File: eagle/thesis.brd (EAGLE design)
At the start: 99.1 x 60.2 mm, 14 parts

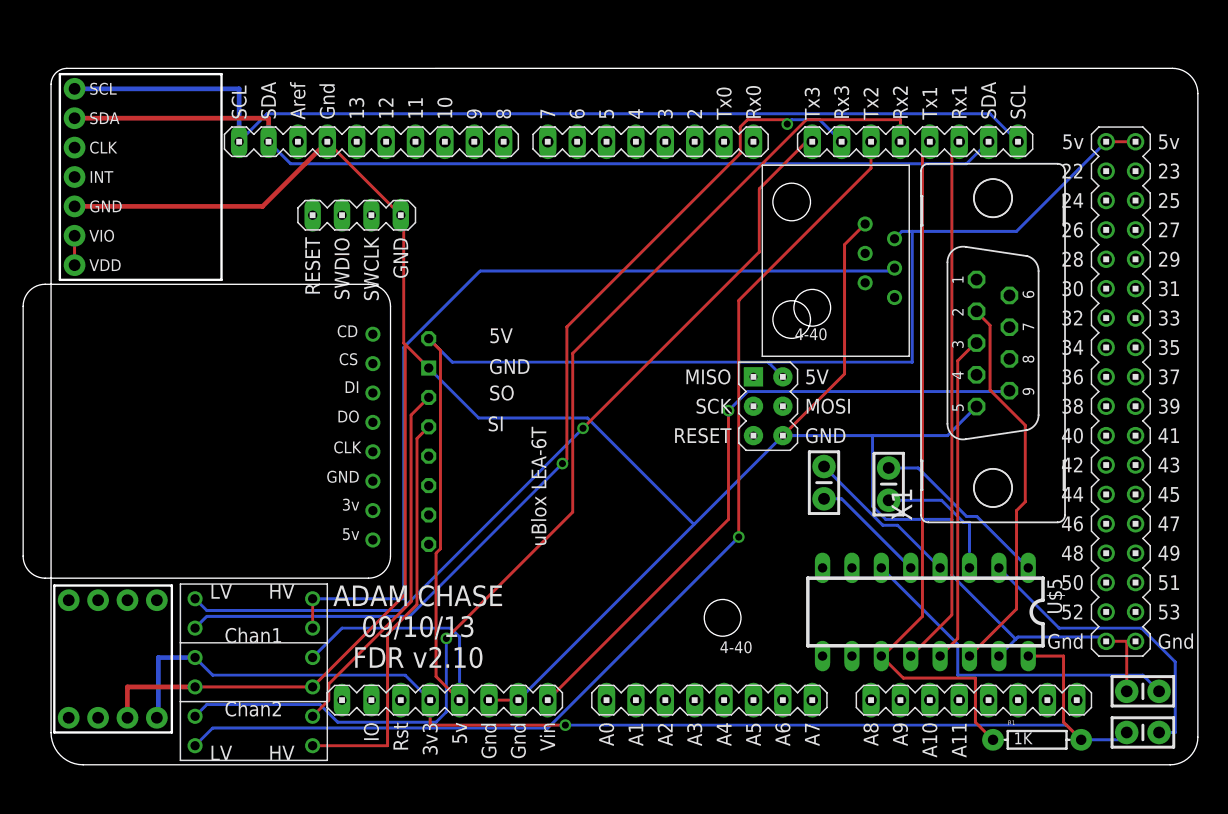
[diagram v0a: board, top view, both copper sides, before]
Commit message: routed thesis board
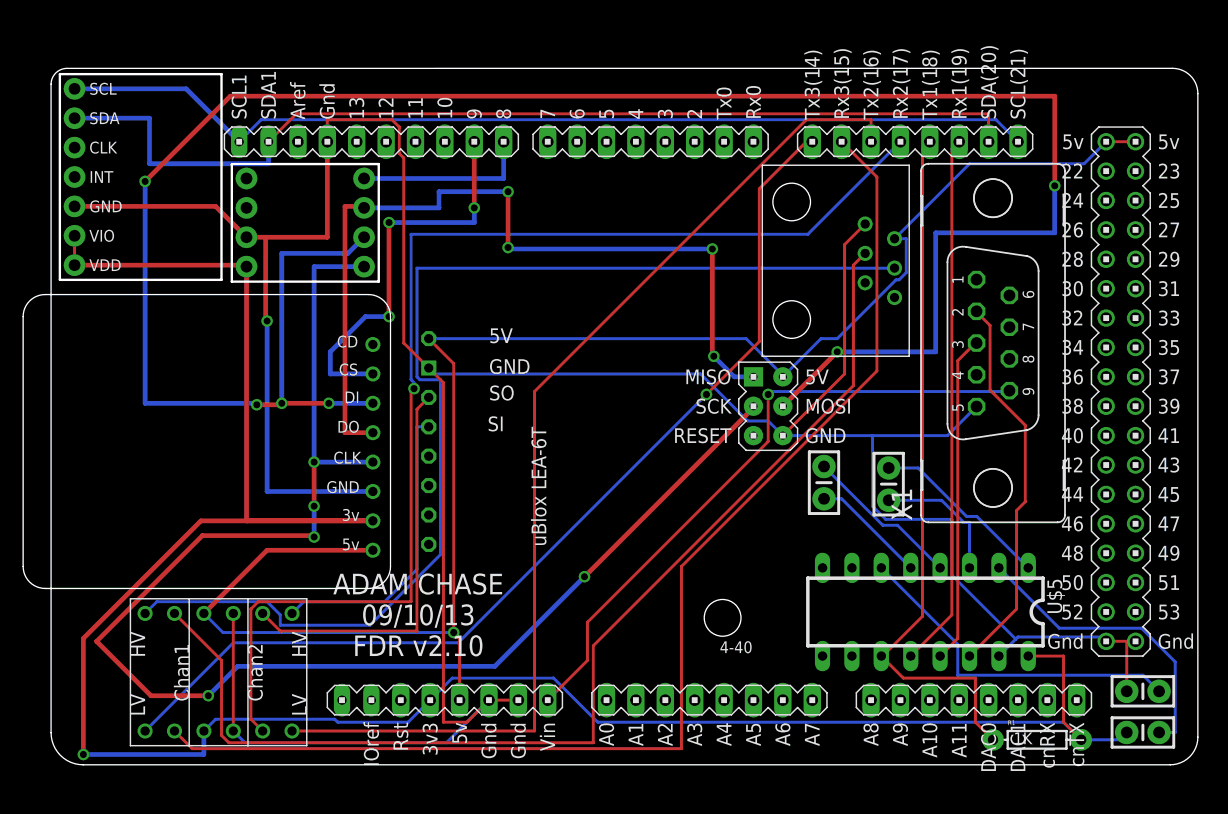
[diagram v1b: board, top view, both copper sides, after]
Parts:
- moved U$4 46.0 mm to (28.3, 51.9), turned to 180 degrees
- moved U$2 11.0 mm to (22.1, 1.65), turned to 90 degrees
- moved U$3 0.89 mm to (-2.67, 14.7)
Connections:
- new net D52: U$1.52
- new net D53: U$1.53
- net ACCELCS: now also U$1.8; no longer U$1.53
- net GND: no longer U$1.GND_DEBUG
- net RX3H: now also U$2.P$11
- net SDCS: now also U$1.9; no longer U$1.52
- net TX3H: no longer U$2.P$11
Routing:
- net MOSI: track 0.00 -> 189.0 mm, vias 0 -> 6
- net SCLK: track 0.00 -> 124.6 mm, vias 0 -> 5
- net RX3H: track 0.00 -> 96.6 mm
- net 3V3: track 107.0 -> 197.4 mm
- net MISO: track 0.00 -> 73.8 mm, vias 0 -> 4
- net GND: track 244.3 -> 280.4 mm, vias 0 -> 1
- net SDCS: track 0.00 -> 34.4 mm, vias 0 -> 3
- net RX3: track 83.4 -> 105.2 mm, vias 2 -> 0
- net TX3H: track 77.4 -> 97.8 mm
- net ACCELCS: track 0.00 -> 15.2 mm
- net 5V: track 132.2 -> 146.2 mm, vias 0 -> 1
- net TX3: track 73.7 -> 86.5 mm
- net TX2H: track 35.5 -> 25.7 mm
- net SDA2: track 82.6 -> 88.6 mm
- net RX2: track 97.2 -> 102.6 mm
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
